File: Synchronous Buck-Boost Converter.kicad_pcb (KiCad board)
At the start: 2 copper layers, 102 x 60 mm, 12 parts, among them J1 Conn_01x06_Pin, Q1 NMOS, Q2 NMOS, Q3 NMOS, Q4 NMOS, U1 IR2110, U2 STM32G4A1CETx, U3 INA240A3D

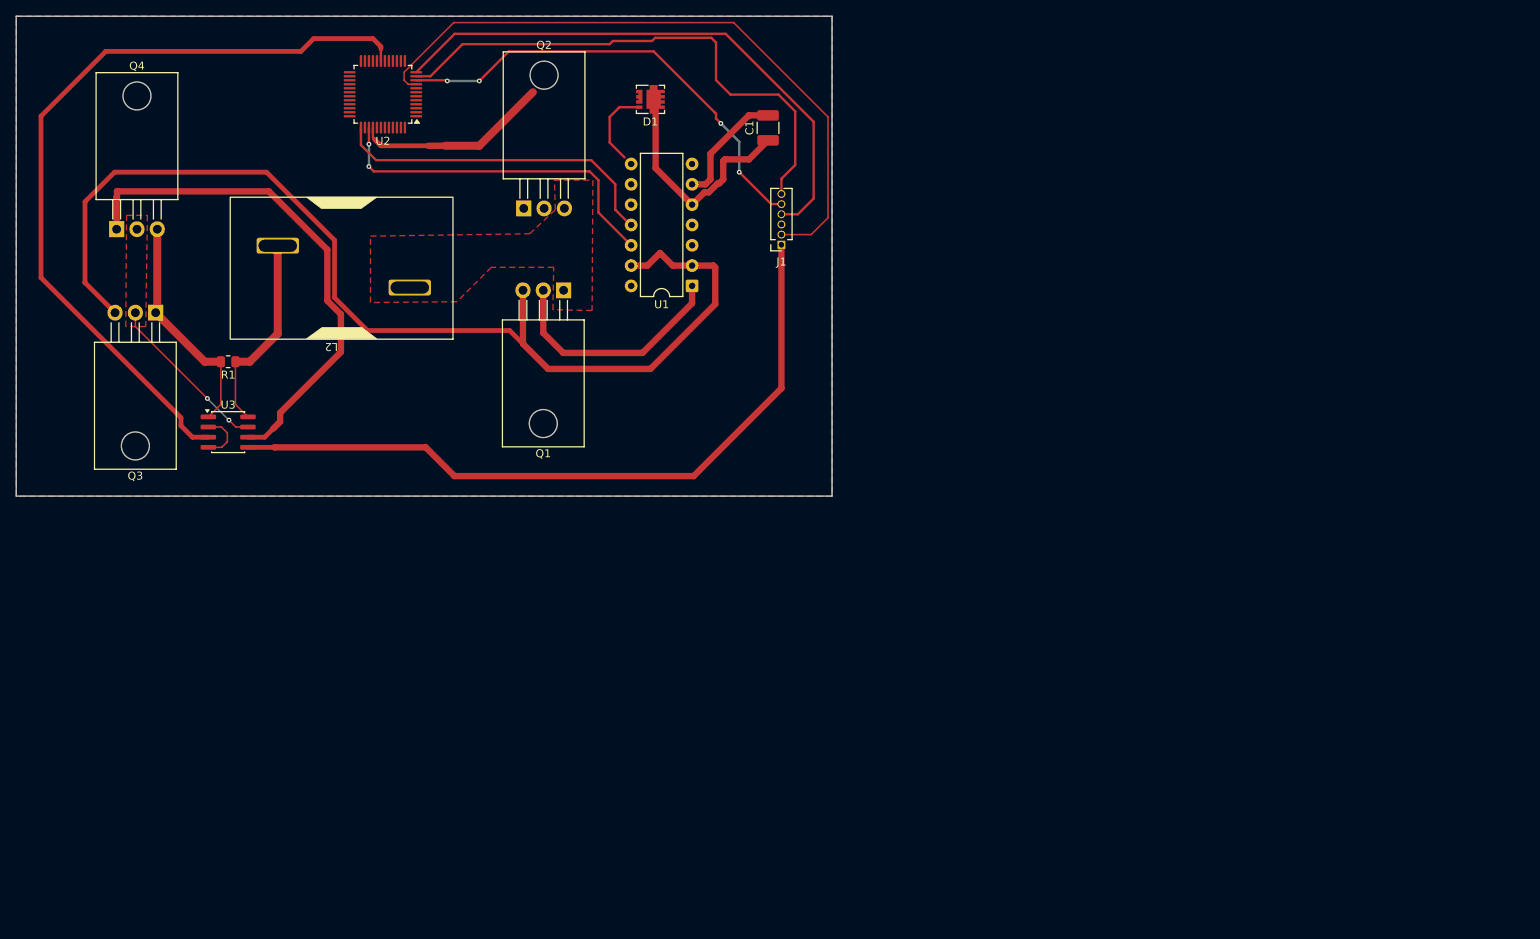
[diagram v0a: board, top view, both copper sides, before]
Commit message: Bidirectionnal Sychronous 4 Switch BB Hardware V1
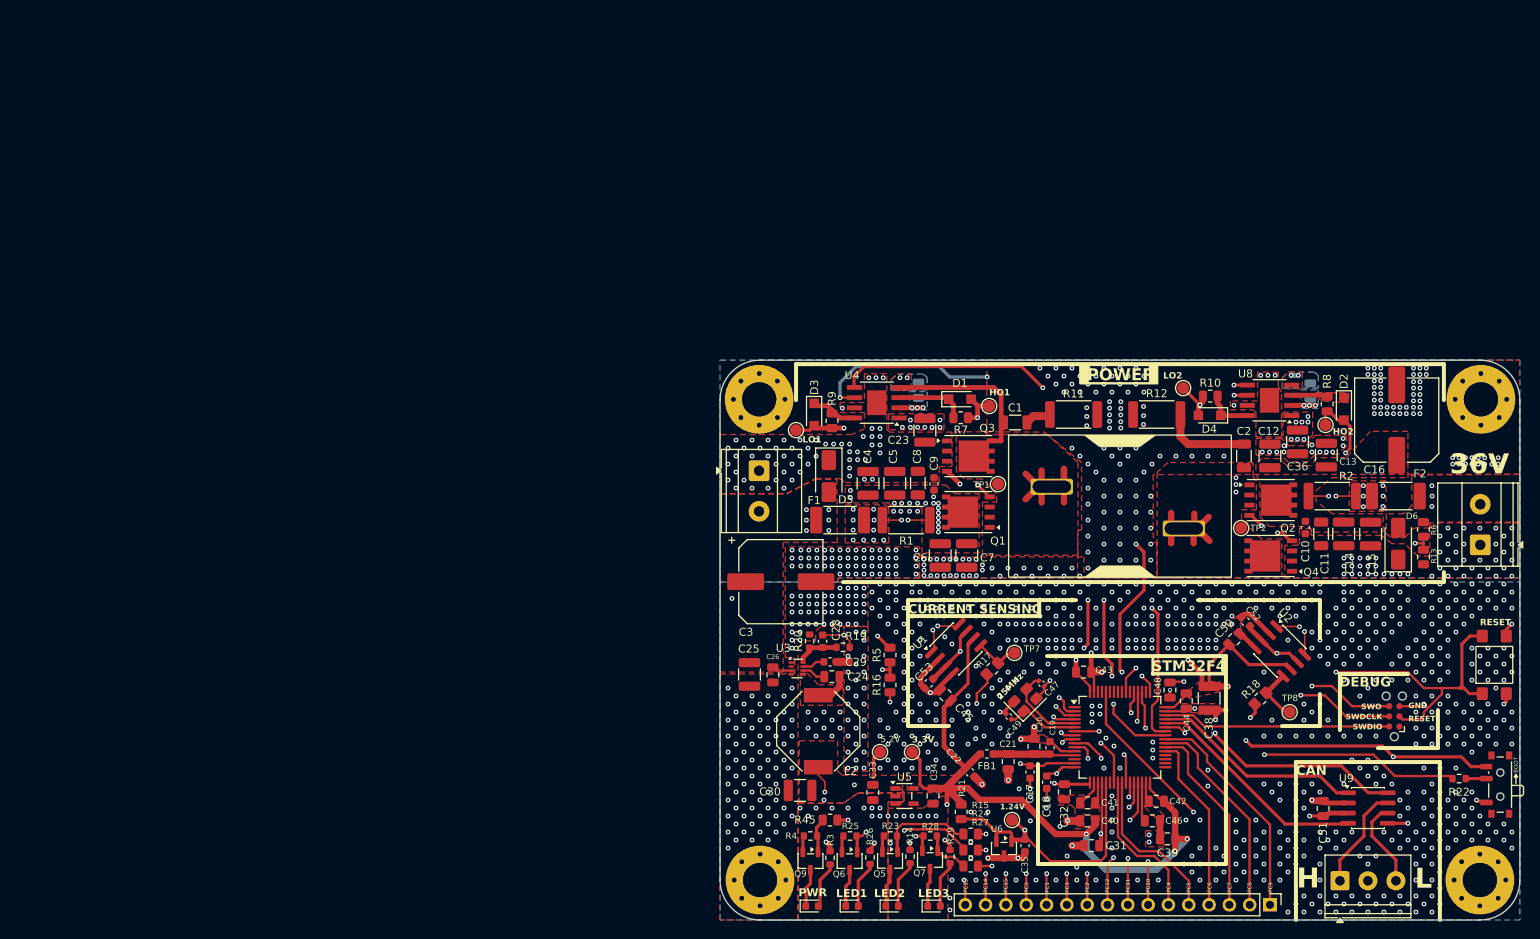
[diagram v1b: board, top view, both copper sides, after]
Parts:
- added C10: 0.1u, Capacitor_SMD:C_0603_1608Metric, F.Cu at (161.2, 63.9)
- added C11: 1u, Capacitor_SMD:C_1206_3216Metric, F.Cu at (163.2, 64.7)
- added C12: 4.7u, Capacitor_SMD:C_1210_3225Metric, F.Cu at (156.8, 55.0)
- added C13: 10u, Capacitor_SMD:C_1210_3225Metric, F.Cu at (163.8, 54.9)
- added C14: 10u, Capacitor_SMD:C_1210_3225Metric, F.Cu at (166.0, 64.7)
- added C15: 10u, Capacitor_SMD:C_1210_3225Metric, F.Cu at (169.3, 64.7)
- added C16: 100u, Capacitor_SMD:C_Elec_10x10.2, F.Cu at (172.6, 50.5)
- added C17: 1n, Capacitor_SMD:C_0603_1608Metric, F.Cu at (126.8, 94.5)
- added C18: 1n, Capacitor_SMD:C_0603_1608Metric, F.Cu at (128.8, 95.8)
- added C19: 10n, Capacitor_SMD:C_0603_1608Metric, F.Cu at (129.2, 91.5)
- added C2: 5.6n, Capacitor_SMD:C_1206_3216Metric, F.Cu at (153.5, 55.0)
- added C20: 100n, Capacitor_SMD:C_0805_2012Metric, F.Cu at (127.2, 91.3)
- added C21: 1u, Capacitor_SMD:C_0805_2012Metric, F.Cu at (124.0, 93.2)
- added C22: 1n, Capacitor_SMD:C_0603_1608Metric, F.Cu at (119.2, 94.5)
- added C23: 10u, Capacitor_SMD:C_1210_3225Metric, F.Cu at (113.6, 51.8)
- added C24: 100n, Capacitor_SMD:C_0805_2012Metric, F.Cu at (102.0, 82.6)
- added C25: 10u, Capacitor_SMD:C_1210_3225Metric, F.Cu at (91.7, 82.3)
- added C26: 100n, Capacitor_SMD:C_0805_2012Metric, F.Cu at (94.6, 82.3)
- added C27: 2.2u, Capacitor_SMD:C_0805_2012Metric, B.Cu at (112.8, 46.8)
- added C28: 12p, Capacitor_SMD:C_0603_1608Metric, F.Cu at (100.8, 78.2)
- added C29: 33n, Capacitor_SMD:C_0603_1608Metric, F.Cu at (101.8, 80.7)
- added C3: 100u, Capacitor_SMD:C_Elec_10x10.2, F.Cu at (95.6, 70.7)
- added C30: 47u, Capacitor_SMD:C_1210_3225Metric, F.Cu at (98.0, 96.8)
- added C31: 100n, Capacitor_SMD:C_0805_2012Metric, F.Cu at (134.4, 103.7)
- added C32: 100n, Capacitor_SMD:C_0805_2012Metric, F.Cu at (131.1, 97.0)
- added C33: 1u, Capacitor_SMD:C_0805_2012Metric, F.Cu at (107.1, 97.0)
- added C34: 1u, Capacitor_SMD:C_0805_2012Metric, F.Cu at (114.6, 97.5)
- added C35: 10n, Capacitor_SMD:C_0603_1608Metric, F.Cu at (126.1, 103.7)
- added C36: 10u, Capacitor_SMD:C_1210_3225Metric, F.Cu at (160.2, 53.2)
- added C37: 2.2u, Capacitor_SMD:C_0805_2012Metric, B.Cu at (161.8, 46.9)
- added C38: 10u, Capacitor_SMD:C_1210_3225Metric, F.Cu at (149.2, 85.3)
- added C39: 4.7u, Capacitor_SMD:C_0805_2012Metric, F.Cu at (143.9, 102.9)
- added C4: 10u, Capacitor_SMD:C_1210_3225Metric, F.Cu at (106.5, 58.4)
- added C40: 4.7u, Capacitor_SMD:C_0805_2012Metric, F.Cu at (133.9, 100.6)
- added C41: 100n, Capacitor_SMD:C_0805_2012Metric, F.Cu at (133.9, 98.3)
- added C42: 100n, Capacitor_SMD:C_0805_2012Metric, F.Cu at (142.6, 98.2)
- added C43: 100n, Capacitor_SMD:C_0805_2012Metric, F.Cu at (133.4, 82.0)
- added C44: 100n, Capacitor_SMD:C_0805_2012Metric, F.Cu at (146.3, 85.6)
- added C45: 100n, Capacitor_SMD:C_0805_2012Metric, F.Cu at (116.2, 84.9)
- added C46: 4.7u, Capacitor_SMD:C_0805_2012Metric, F.Cu at (142.1, 100.6)
- added C47: 18p, Capacitor_SMD:C_0402_1005Metric, F.Cu at (128.2, 83.5)
- added C48: 100n, Capacitor_SMD:C_0805_2012Metric, F.Cu at (144.2, 84.2)
- added C49: 18p, Capacitor_SMD:C_0402_1005Metric, F.Cu at (124.1, 87.6)
- added C5: 10u, Capacitor_SMD:C_1210_3225Metric, F.Cu at (109.8, 58.4)
- added C50: 100n, Capacitor_SMD:C_0805_2012Metric, F.Cu at (152.3, 77.9)
- added C51: 100n, Capacitor_SMD:C_0805_2012Metric, F.Cu at (163.4, 99.0)
- added C52: 10n, Capacitor_SMD:C_0603_1608Metric, F.Cu at (153.7, 75.7)
- added C53: 10n, Capacitor_SMD:C_0603_1608Metric, F.Cu at (114.1, 83.4)
- added C6: 10u, Capacitor_SMD:C_1210_3225Metric, F.Cu at (115.5, 67.4)
- added C7: 4.7u, Capacitor_SMD:C_1210_3225Metric, F.Cu at (118.8, 67.4)
- added C8: 1u, Capacitor_SMD:C_1206_3216Metric, F.Cu at (112.7, 58.4)
- added C9: 0.1u, Capacitor_SMD:C_0603_1608Metric, F.Cu at (114.8, 58.5)
- added D10: GREEN LED, LED_SMD:LED_0603_1608Metric, F.Cu at (99.5, 111.2)
- added D11: RED LED, LED_SMD:LED_0603_1608Metric, F.Cu at (104.5, 111.2)
- added D12: GREEN LED, LED_SMD:LED_0603_1608Metric, F.Cu at (114.8, 111.2)
- added D2: SKL16, Diode_SMD:Nexperia_CFP3_SOD-123W, F.Cu at (166.0, 49.1)
- added D3: SKL16, Diode_SMD:Nexperia_CFP3_SOD-123W, F.Cu at (99.8, 49.8)
- added D4: SKL16, Diode_SMD:Nexperia_CFP3_SOD-123W, F.Cu at (149.2, 49.9)
- added D5: 70V, Diode_SMD:D_SMA, F.Cu at (101.6, 57.5)
- added D6: 70V, Diode_SMD:D_SMA, F.Cu at (172.8, 66.0)
- added D9: YELLOW LED, LED_SMD:LED_0603_1608Metric, F.Cu at (109.5, 111.2)
- added F1: 15A, Fuse:Fuse_2512_6332Metric_Pad1.52x3.35mm_HandSolder, F.Cu at (103.0, 63.0)
- added F2: 15A, Fuse:Fuse_2512_6332Metric_Pad1.52x3.35mm_HandSolder, F.Cu at (172.5, 60.0)
- added FB1: 600R, Inductor_SMD:L_0603_1608Metric, F.Cu at (121.4, 92.2)
- added H1: MountingHole_Pad, MountingHole:MountingHole_4.3mm_M4_Pad_Via, F.Cu at (92.9, 47.9)
- added H2: MountingHole_Pad, MountingHole:MountingHole_4.3mm_M4_Pad_Via, F.Cu at (183.1, 47.9)
- added H3: MountingHole_Pad, MountingHole:MountingHole_4.3mm_M4_Pad_Via, F.Cu at (183.0, 108.0)
- added H4: MountingHole_Pad, MountingHole:MountingHole_4.3mm_M4_Pad_Via, F.Cu at (93.0, 108.0)
- added J2: Screw_Terminal_01x02, TerminalBlock_Phoenix:TerminalBlock_Phoenix_MKDS-1,5-2-5.08_1x02_P5.08mm_Horizontal, F.Cu at (183.1, 66.1)
- added J3: Screw_Terminal_01x03, TerminalBlock_Phoenix:TerminalBlock_Phoenix_PT-1,5-3-3.5-H_1x03_P3.50mm_Horizontal, F.Cu at (165.5, 108.1)
- added J4: Conn_01x16_Pin, Connector_PinHeader_2.54mm:PinHeader_1x16_P2.54mm_Vertical, F.Cu at (156.8, 111.1)
- added J6: Conn_ARM_SWD_TagConnect_TC2030-NL, Connector:Tag-Connect_TC2030-IDC-NL_2x03_P1.27mm_Vertical, F.Cu at (172.3, 87.5)
- added L1: VER2923-22uH, Power_Inductor_THT:VER2923, F.Cu at (129.5, 58.8)
- added Q5: BSR14, Package_TO_SOT_SMD:SOT-23-3, F.Cu at (109.2, 105.6)
- added Q6: BSR14, Package_TO_SOT_SMD:SOT-23-3, F.Cu at (104.2, 105.6)
- added Q7: BSR14, Package_TO_SOT_SMD:SOT-23-3, F.Cu at (114.2, 105.5)
- added Q9: BSR14, Package_TO_SOT_SMD:SOT-23-3, F.Cu at (99.3, 105.6)
- added R10: 5.11, Resistor_SMD:R_0805_2012Metric, F.Cu at (149.3, 47.5)
- added R11: 3.3, Resistor_SMD:R_2512_6332Metric, F.Cu at (132.2, 49.8)
- added R12: 3.3, Resistor_SMD:R_2512_6332Metric, F.Cu at (142.6, 49.8)
- added R13: 4k7R, Resistor_SMD:R_0805_2012Metric, F.Cu at (175.9, 67.6)
- added R14: 470, Resistor_SMD:R_0603_1608Metric, F.Cu at (111.8, 105.1)
- added R15: 4k7R, Resistor_SMD:R_0805_2012Metric, F.Cu at (119.3, 102.2)
- added R16: 4k7R, Resistor_SMD:R_0805_2012Metric, F.Cu at (109.2, 83.6)
- added R17: 1kR, Resistor_SMD:R_0805_2012Metric_Pad1.20x1.40mm_HandSolder, F.Cu at (122.0, 81.6)
- added R18: 1kR, Resistor_SMD:R_0805_2012Metric_Pad1.20x1.40mm_HandSolder, F.Cu at (155.6, 85.3)
- added R19: 54.9k, Resistor_SMD:R_0603_1608Metric, F.Cu at (103.4, 78.9)
- added R2: 0.003, Resistor_SMD:R_2512_6332Metric, F.Cu at (164.5, 60.0)
- added R20: 10k, Resistor_SMD:R_0603_1608Metric, F.Cu at (99.2, 78.1)
- added R21: 200, Resistor_SMD:R_0805_2012Metric, F.Cu at (118.2, 99.5)
- added R22: 10k, Resistor_SMD:R_0603_1608Metric, F.Cu at (180.4, 95.3)
- added R23: 10k, Resistor_SMD:R_0603_1608Metric, F.Cu at (109.3, 102.5)
- added R24: 4k7R, Resistor_SMD:R_0805_2012Metric, F.Cu at (119.3, 104.2)
- added R25: 10k, Resistor_SMD:R_0603_1608Metric, F.Cu at (104.2, 102.5)
- added R26: 390, Resistor_SMD:R_0603_1608Metric, F.Cu at (106.8, 105.2)
- added R27: 4k7R, Resistor_SMD:R_0805_2012Metric, F.Cu at (119.3, 106.2)
- added R28: 10k, Resistor_SMD:R_0603_1608Metric, F.Cu at (114.3, 102.5)
- added R29: 270, Resistor_SMD:R_0603_1608Metric, F.Cu at (116.8, 105.1)
- added R3: 470, Resistor_SMD:R_0603_1608Metric, F.Cu at (101.8, 105.2)
- added R4: 10k, Resistor_SMD:R_0603_1608Metric, F.Cu at (99.3, 102.5)
- added R45: 4k7R, Resistor_SMD:R_0805_2012Metric, F.Cu at (101.8, 100.5)
- added R5: 51kR, Resistor_SMD:R_0805_2012Metric, F.Cu at (109.2, 79.9)
- added R6: 51kR, Resistor_SMD:R_0805_2012Metric, F.Cu at (175.9, 64.2)
- added R7: 5.11, Resistor_SMD:R_0805_2012Metric, F.Cu at (118.1, 50.2)
- added R8: 5.11, Resistor_SMD:R_0805_2012Metric, F.Cu at (163.9, 48.5)
- added R9: 5.11, Resistor_SMD:R_0805_2012Metric, F.Cu at (102.0, 50.6)
- added SW1: TL3305, Button:TL3305, F.Cu at (184.8, 81.1)
- added SW2: SW_SPDT, Button_Switch_SMD:SW_SPDT_PCM12, F.Cu at (185.2, 96.1)
- added TP1: ~, TestPoint:TestPoint_Pad_D1.5mm, F.Cu at (122.8, 58.5)
- added TP12: +3.3V, TestPoint:TestPoint_Pad_D1.5mm, F.Cu at (112.0, 92.0)
- added TP13: +1.24V, TestPoint:TestPoint_Pad_D1.5mm, F.Cu at (124.5, 100.5)
- added TP2: ~, TestPoint:TestPoint_Pad_D1.5mm, F.Cu at (153.2, 64.0)
- added TP3: ~, TestPoint:TestPoint_Pad_D1.5mm, F.Cu at (121.6, 48.7)
- added TP4: ~, TestPoint:TestPoint_Pad_D1.5mm, F.Cu at (163.7, 51.1)
- added TP5: ~, TestPoint:TestPoint_Pad_D1.5mm, F.Cu at (97.5, 51.8)
- added TP6: ~, TestPoint:TestPoint_Pad_D1.5mm, F.Cu at (145.9, 46.5)
- added TP7: ~, TestPoint:TestPoint_Pad_D1.5mm, F.Cu at (124.8, 79.6)
- added TP8: ~, TestPoint:TestPoint_Pad_D1.5mm, F.Cu at (159.2, 87.0)
- added TP9: 5.2V, TestPoint:TestPoint_Pad_D1.5mm, F.Cu at (108.0, 92.0)
- added U4: UCC27211A, Package_SO:TI_SO-PowerPAD-8, F.Cu at (107.6, 48.3)
- added U5: MIC5504-3.3YM5, Package_TO_SOT_SMD:SOT-23-5, F.Cu at (111.1, 97.5)
- added U6: TLV431, Package_TO_SOT_SMD:SOT-23, F.Cu at (123.5, 104.1)
- added U7: STM32F446RETx, Package_QFP:LQFP-64_10x10mm_P0.5mm, F.Cu at (138.0, 90.2)
- added U8: UCC27211A, Package_SO:TI_SO-PowerPAD-8, F.Cu at (156.7, 48.0)
- added U9: TJA1051T-3, Package_SO:SOIC-8_3.9x4.9mm_P1.27mm, F.Cu at (169.0, 99.0)
- added Y1: 25MHz, Crystal:Crystal_SMD_3225-4Pin_3.2x2.5mm, F.Cu at (126.2, 85.5)
- C1: value C -> 5.6n; footprint Capacitor_SMD:C_1210_3225Metric_Pad1.33x2.70mm_HandSolder -> Capacitor_SMD:C_1206_3216Metric
- D1: value D -> SKL16; footprint Diode_SMD:D_QFN_3.3x3.3mm_P0.65mm -> Diode_SMD:Nexperia_CFP3_SOD-123W
- J1: value Conn_01x06_Pin -> Screw_Terminal_01x02; footprint Connector_PinSocket_1.27mm:PinSocket_1x06_P1.27mm_Vertical -> TerminalBlock_Phoenix:TerminalBlock_Phoenix_MKDS-1,5-2-5.08_1x02_P5.08mm_Horizontal
- L2: value VER2923-22uH -> 5.2uH; footprint Power_Inductor:VER2923 -> Power_Inductor_THT:L_Bourns-SRU1038_10.0x10.0mm
- Q1, Q2, Q3, Q4: value NMOS -> SiR182DP; footprint Package_TO_SOT_THT:TO-220-3_Horizontal_TabDown -> Mosfets:PowerPAK_SO-8_Single
- R1: value R -> 0.003; footprint Resistor_SMD:R_0805_2012Metric -> Resistor_SMD:R_2512_6332Metric
- U1: value IR2110 -> INA240A1; footprint Package_DIP:DIP-14_W7.62mm -> Package_SO:SOIC-8_3.9x4.9mm_P1.27mm
- U2: value STM32G4A1CETx -> INA240A1; footprint Package_QFP:LQFP-48_7x7mm_P0.5mm -> Package_SO:SOIC-8_3.9x4.9mm_P1.27mm
- U3: value INA240A3D -> TPS62932; footprint Package_SO:SOIC-8_3.9x4.9mm_P1.27mm -> Package_TO_SOT_SMD:SOT-583-8
- moved Q4 150.0 mm to (156.8, 67.5), turned to 180 degrees
- moved U2 132.0 mm to (158.0, 79.4), turned to -45 degrees
- moved Q3 103.2 mm to (119.0, 55.0), turned to 0 degrees
- moved Q2 100.3 mm to (156.9, 60.5)
- moved R1 87.0 mm to (111.3, 63.0), turned to 0 degrees
- moved U3 77.0 mm to (97.6, 81.6)
- moved L2 75.4 mm to (100.3, 89.4), turned to -90 degrees
- moved Q1 57.7 mm to (119.0, 62.0)
- moved U1 56.1 mm to (117.5, 79.1), turned to 45 degrees
- moved D1 53.9 mm to (118.0, 47.9), turned to 0 degrees
- moved C1 48.1 mm to (124.9, 50.8), turned to 0 degrees
- moved J1 28.4 mm to (92.9, 56.8), turned to -90 degrees
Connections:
- C1 pad 1: Net-(D1-K) -> SW1
- C1 pad 2: Net-(U1-VB) -> Net-(C1-Pad2)
- D1 pad 1: Net-(D1-K) -> HO_1
- J1 pad 1: Net-(J1-Pin_1) -> GND
- J1 pad 2: Net-(J1-Pin_2) -> +12V
- L2 pad 1: Net-(Q1-D) -> Net-(U3-SW)
- L2 pad 2: Net-(U3-+) -> +5.2V
- Q1 pad 1: Net-(Q1-D) -> SW1
- Q1 pad 2: Net-(Q1-G) -> SW1
- Q1 pad 3: Net-(Q1-S) -> SW1
- Q2 pad 1: Net-(J1-Pin_3) -> SW2
- Q2 pad 2: Net-(Q2-G) -> SW2
- Q2 pad 3: Net-(Q1-D) -> SW2
- Q3 pad 1: Net-(Q3-D) -> GND
- Q3 pad 2: Net-(Q3-G) -> GND
- Q3 pad 3: Net-(Q1-S) -> GND
- Q4 pad 1: Net-(J1-Pin_3) -> GND
- Q4 pad 2: Net-(Q3-G) -> GND
- Q4 pad 3: Net-(Q3-D) -> GND
- R1 pad 1: Net-(U3-+) -> +12V
- R1 pad 2: Net-(Q3-D) -> +12V
- U1 pad 1: Net-(Q1-G) -> +12V
- U1 pad 2: Net-(Q1-S) -> GND
- U1 pad 3: Net-(J1-Pin_3) -> +Vref
- U1 pad 4: unconnected-(U1-NC-Pad4) -> GND
- U1 pad 5: Net-(D1-K) -> Net-(R17-Pad1)
- U1 pad 6: Net-(U1-VB) -> +3.3V
- U1 pad 7: Net-(Q2-G) -> +Vref
- U1 pad 8: unconnected-(U1-NC-Pad8) -> +12V
- U2 pad 1: unconnected-(U2-VBAT-Pad1) -> +36V
- U2 pad 2: unconnected-(U2-PC13-Pad2) -> GND
- U2 pad 3: unconnected-(U2-PC14-Pad3) -> +Vref
- U2 pad 4: unconnected-(U2-PC15-Pad4) -> GND
- U2 pad 5: unconnected-(U2-PF0-Pad5) -> Net-(R18-Pad2)
- U2 pad 6: unconnected-(U2-PF1-Pad6) -> +3.3V
- U2 pad 7: unconnected-(U2-PG10-Pad7) -> +Vref
- U2 pad 8: unconnected-(U2-PA0-Pad8) -> +36V
- U3 pad 1: Net-(Q3-D) -> unconnected-(U3-RT-Pad1)
- U3 pad 2: GND -> unconnected-(U3-EN-Pad2)
- U3 pad 3: Net-(U2-VSSA) -> +12V
- U3 pad 5: Net-(J1-Pin_1) -> Net-(U3-SW)
- U3 pad 6: Net-(J1-Pin_3) -> Net-(U3-BST)
- U3 pad 7: Net-(Q3-G) -> Net-(U3-SS)
- U3 pad 8: Net-(U3-+) -> Net-(U3-FB)
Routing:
- net +3.3V: track 0.00 -> 232.1 mm, vias 0 -> 14
- net Net-(Q1-S): track 136.7 -> 0.00 mm
- net +5.2V: track 0.00 -> 127.9 mm, vias 0 -> 6
- net +12V: track 0.00 -> 117.6 mm, vias 0 -> 53
- net +Vref: track 0.00 -> 117.5 mm, vias 0 -> 3
- net Net-(U2-VSSA): track 98.7 -> 0.00 mm
- net Net-(J1-Pin_1): track 90.7 -> 0.00 mm
- net GND: track 6.45 -> 95.1 mm, vias 0 -> 1240
- net LI_1: track 0.00 -> 84.0 mm, vias 0 -> 5
- net Net-(J1-Pin_2): track 82.5 -> 0.00 mm
- net HI_1: track 0.00 -> 79.5 mm, vias 0 -> 4
- net V_2: track 0.00 -> 77.3 mm, vias 0 -> 2
- net RESET: track 0.00 -> 74.2 mm, vias 0 -> 3
- net Net-(J1-Pin_4): track 70.7 -> 0.00 mm
- net Net-(J1-Pin_6): track 67.0 -> 0.00 mm
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- added copper zone on F.Cu, net +12V
- added copper zone on In1.Cu, net +12V
- added copper zone on F.Cu, net +3.3V
- added copper zone on F.Cu, net +36V
- added copper zone on F.Cu, net +5.2V
- added copper zone on B.Cu, net GND
- added copper zone on In1.Cu, net GND
- added copper zone on F.Cu, net HO_2
- added copper zone on F.Cu, net Net-(U3-SW)
- added copper zone on B.Cu, net Net-(U4-HB)
- added copper zone on B.Cu, net Net-(U8-HB)
- added copper zone on B.Cu, net SW1
- added copper zone on F.Cu, net SW1
- added copper zone on B.Cu, net SW2
- added copper zone on F.Cu, net SW2
- removed copper zone on F.Cu, net Net-(Q1-D)
- removed copper zone on F.Cu, net Net-(Q3-G)
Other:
- board size 102 x 60 mm -> 100 x 70 mm
- copper layers 2 -> 4
- board text added: "+"
- board text added: "1.24V"
- board text added: "12V"
- board text added: "15A 12V <=> 5A 36V Bidirectionnal Synchronous Buck-Boost Converter 28/06/2026 V1.0 Raphaël Maestri"
- board text added: "25MHz"
- board text added: "3.3V"
- board text added: "36V"
- board text added: "BOOT"
- board text added: "CAN"
- board text added: "CURRENT SENSING"
- board text added: "DEBUG"
- board text added: "GND"
- board text added: "H"
- board text added: "HO1"
- board text added: "HO2"
- board text added: "L"
- board text added: "LED1"
- board text added: "LED2"
- board text added: "LED3"
- board text added: "LO1"
- board text added: "LO2"
- board text added: "PC0"
- board text added: "PC1"
- board text added: "PC10"
- board text added: "PC11"
- board text added: "PC12"
- board text added: "PC13"
- board text added: "PC14"
- board text added: "PC15"
- board text added: "PC2"
- board text added: "PC3"
- board text added: "PC4"
- board text added: "PC5"
- board text added: "PC6"
- board text added: "PC7"
- board text added: "PC8"
- board text added: "PC9"
- board text added: "POWER"
- board text added: "PWR"
- board text added: "RESET"
- board text added: "STM32F4"
- board text added: "SWDCLK"
- board text added: "SWDIO"
- board text added: "SWO"
